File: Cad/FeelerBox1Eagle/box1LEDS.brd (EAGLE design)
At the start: 45 x 70 mm, 13 parts

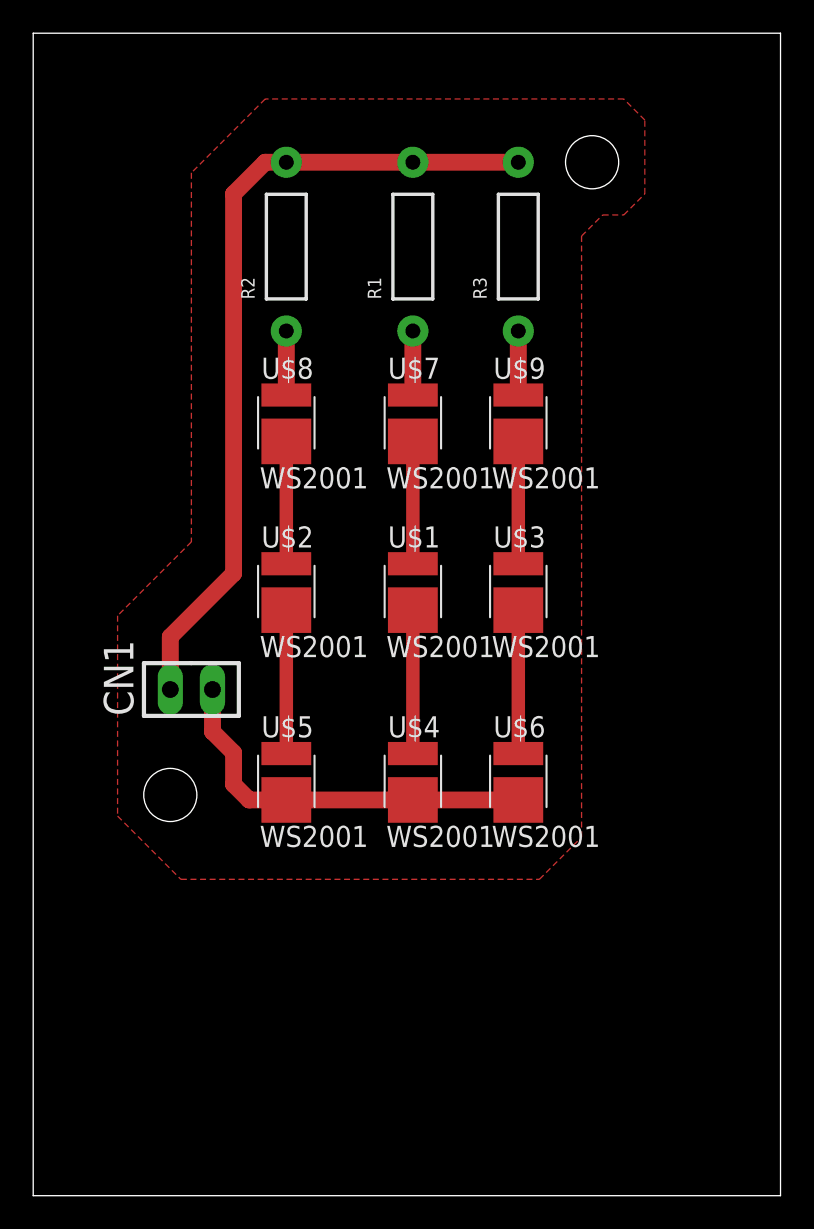
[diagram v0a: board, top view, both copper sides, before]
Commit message: updates
bah
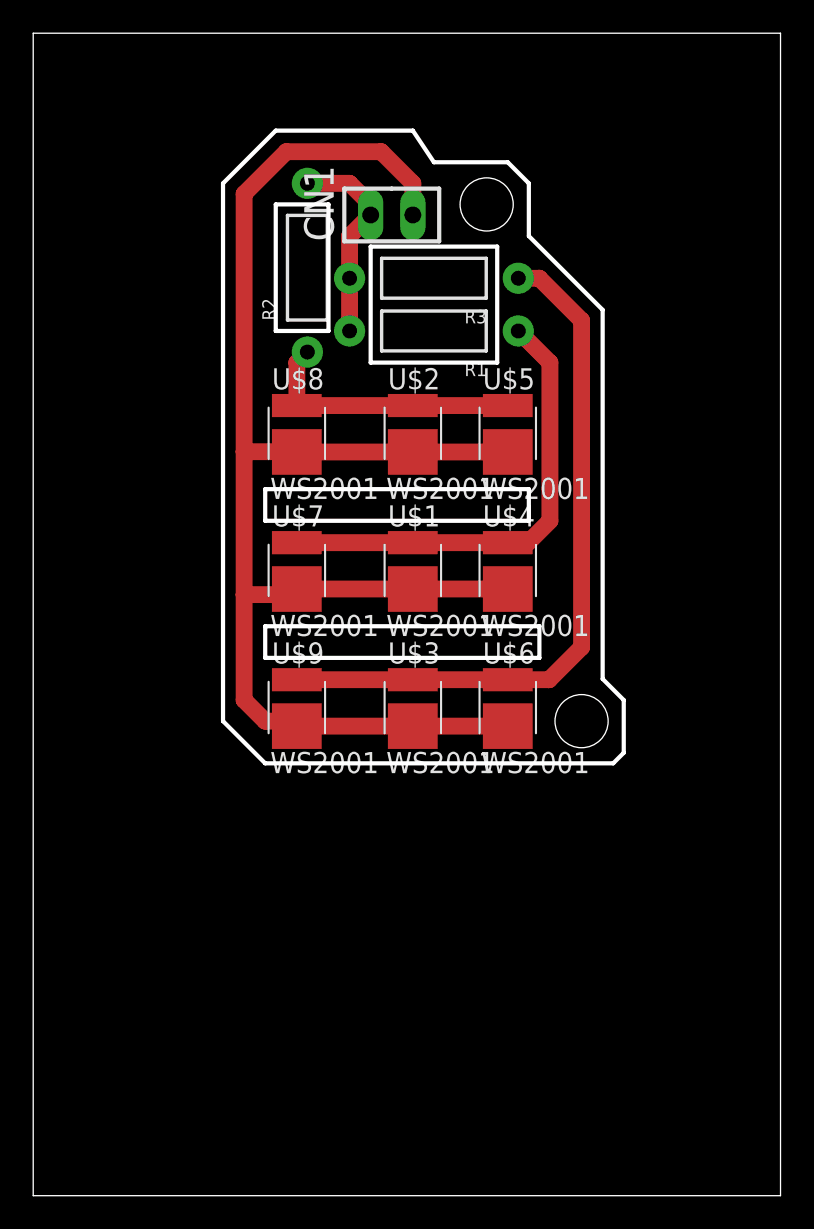
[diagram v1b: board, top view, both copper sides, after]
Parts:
- moved CN1 31.0 mm to (21.6, 59.1)
- moved U$5 24.8 mm to (28.6, 46.4)
- moved U$9 21.7 mm to (15.9, 29.8)
- moved U$4 13.9 mm to (28.6, 38.1)
- moved U$2 12.2 mm to (22.9, 46.4)
- moved U$7 11.3 mm to (15.9, 38.1)
- moved U$3 9.44 mm to (22.9, 29.8)
- moved R3 5.43 mm to (24.1, 55.2), turned to 180 degrees
- moved R1 5.24 mm to (24.1, 52.1), turned to 180 degrees
- moved U$6 4.49 mm to (28.6, 29.8)
- moved R2 1.80 mm to (16.5, 55.9)
- moved U$1 1.27 mm to (22.9, 38.1)
- moved U$8 0.90 mm to (15.9, 46.4)
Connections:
- removed net N$20: U$1.2, U$7.1
- removed net N$21: U$2.2, U$8.1
- removed net N$22: U$3.2, U$9.1
- removed net N$23: U$3.1, U$6.2
- removed net N$24: U$2.1, U$5.2
- removed net N$25: U$1.1, U$4.2
- removed net N$4: CN1.2, U$4.1, U$5.1, U$6.1
- new net GND: CN1.2, U$1.1, U$2.1, U$3.1, U$4.1, U$5.1, U$6.1, U$7.1, U$8.1, U$9.1
- net N$1: now also U$3.2, U$6.2
- net N$2: now also U$2.2, U$5.2
- net N$3: now also U$1.2, U$4.2
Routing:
- net GND: track 0.00 -> 93.9 mm
- net N$1: track 3.86 -> 42.5 mm
- net N$5: track 49.4 -> 12.5 mm
- net N$3: track 3.86 -> 28.0 mm
- net N$4: track 23.8 -> 0.00 mm
- net N$2: track 3.86 -> 16.2 mm
- net N$25: track 8.64 -> 0.00 mm
- net N$24: track 8.64 -> 0.00 mm
- net N$23: track 8.64 -> 0.00 mm
- net N$22: track 7.37 -> 0.00 mm
- net N$21: track 7.37 -> 0.00 mm
- net N$20: track 6.40 -> 0.00 mm
- removed copper zone on layer 1, net N$6
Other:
- outline, holes or cut-outs redrawn
